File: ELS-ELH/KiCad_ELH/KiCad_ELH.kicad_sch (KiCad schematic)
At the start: 18 parts, among them J3 Screw_Terminal_01x12, J4 Screw_Terminal_01x02, J5 Screw_Terminal_01x02, J6 Screw_Terminal_01x02, J7 Screw_Terminal_01x02

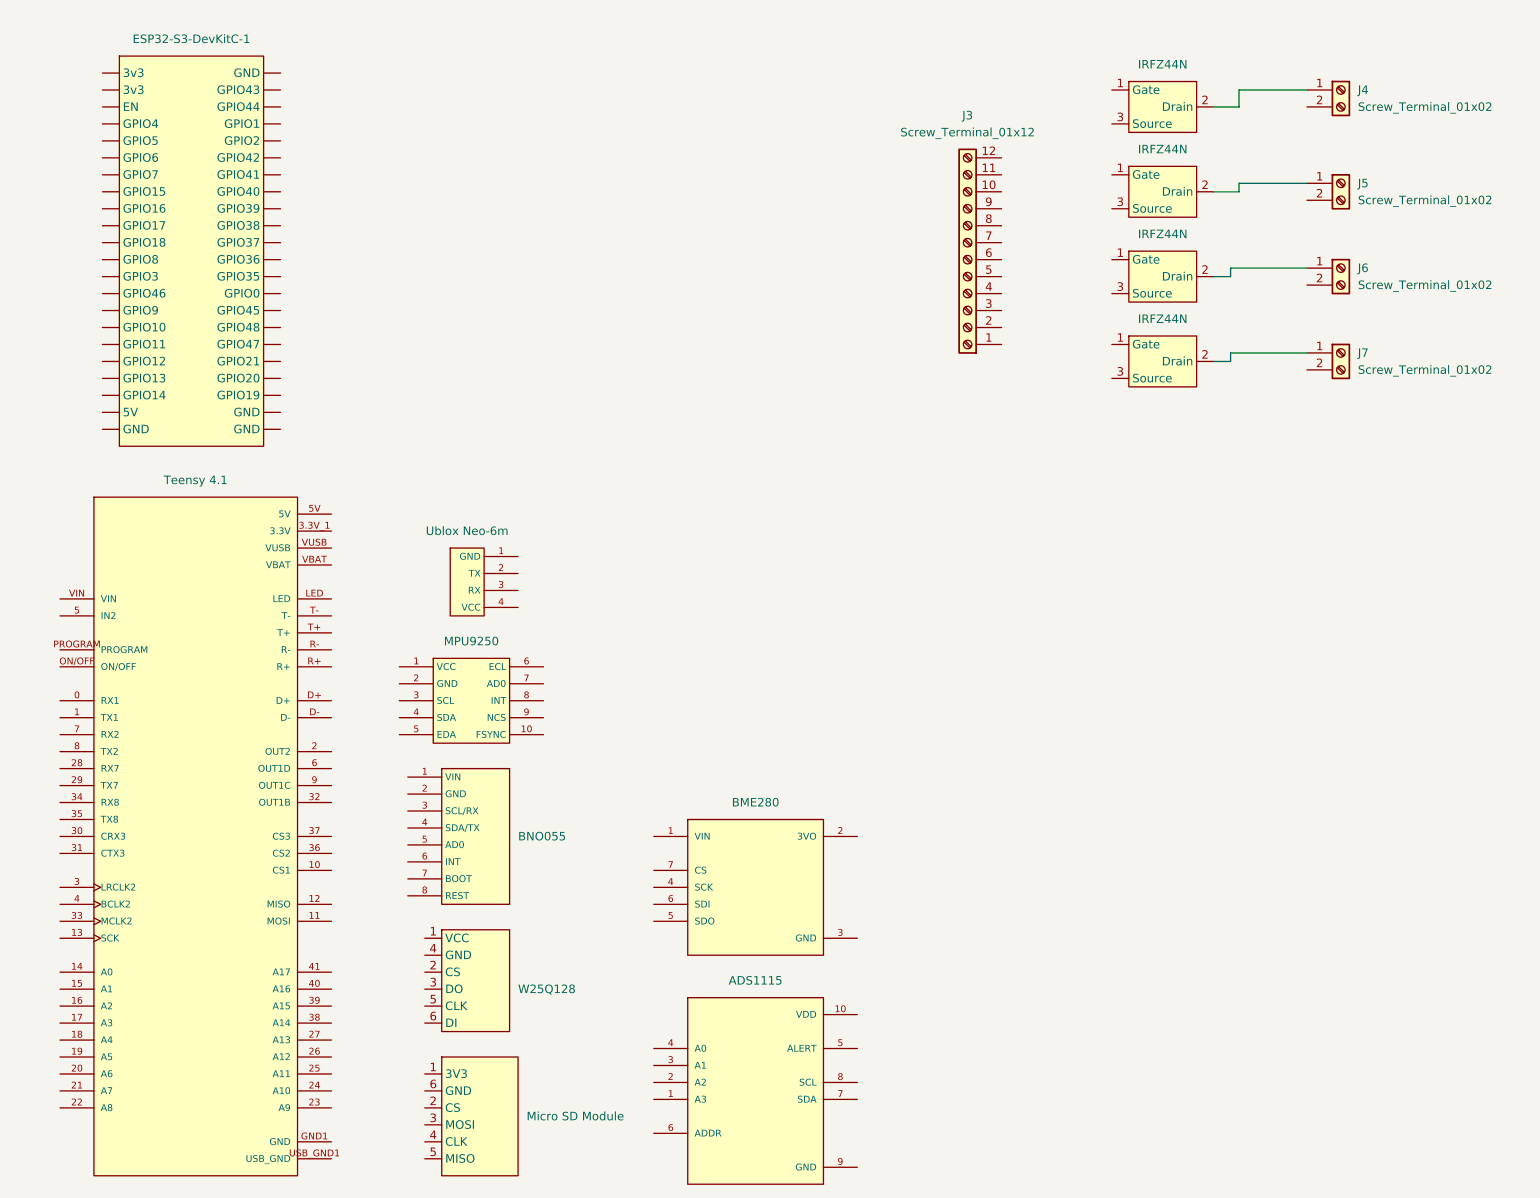
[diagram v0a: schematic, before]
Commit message: Some progress
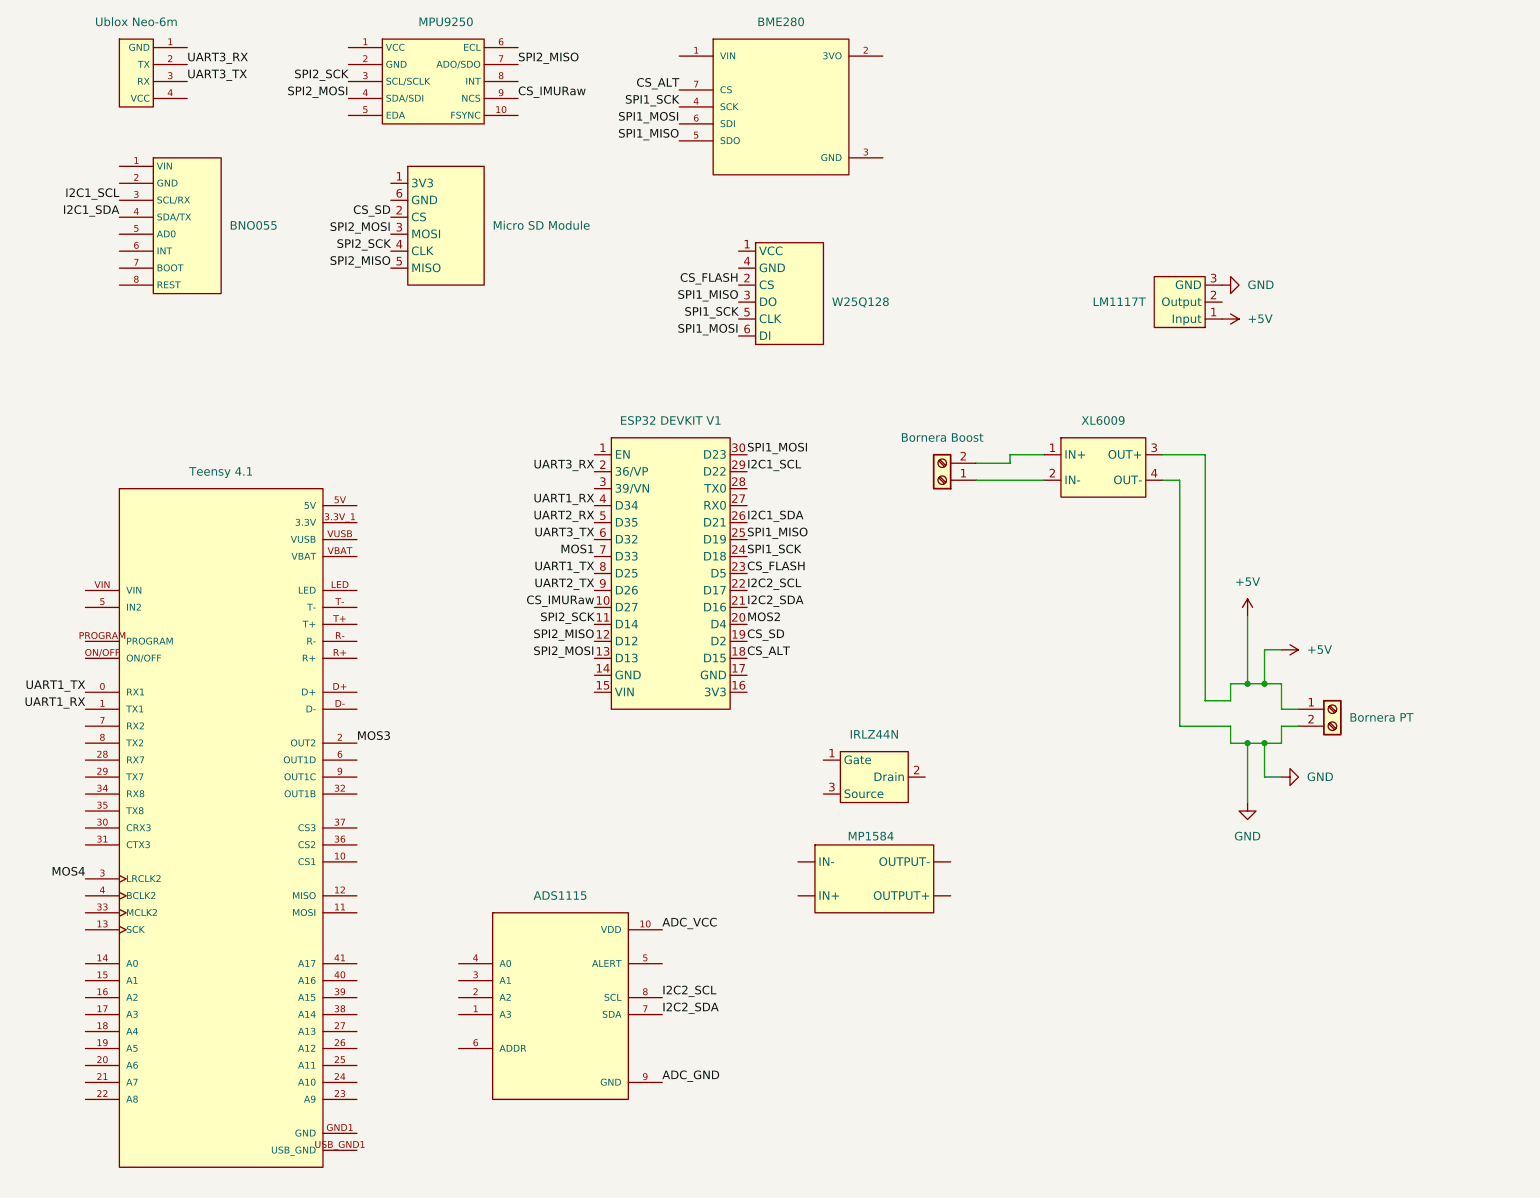
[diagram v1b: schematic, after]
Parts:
- removed ESP32-S3: ESP32-S3-DevKitC-1, ELH_Library:ESP32-S3-DevKitC-1, symbol ELH_Library:ESP32-S3-DevKitC-1
- removed J3: Screw_Terminal_01x12, symbol Connector:Screw_Terminal_01x12
- removed J4, J5, J6, J7: Screw_Terminal_01x02, symbol Connector:Screw_Terminal_01x02
- removed MOSFET1, MOSFET2, MOSFET3, MOSFET5: IRFZ44N, symbol ELH_Library:IRFZ44N
- added BOOST1: XL6009, ELH_Library:XL6009 Boost, symbol ELH_Library:XL6009_Boost
- added Bornera1: Bornera Boost, ELH_Library:Bornera 2P, symbol Connector:Screw_Terminal_01x02
- added Bornera2: Bornera PT, ELH_Library:Bornera 2P, symbol Connector:Screw_Terminal_01x02
- added ESP1: ESP32 DEVKIT V1, ELH_Library:ESP32 DEVKIT V1, symbol ELH_Library:ESP32 DEVKIT V1
- added MOSFET1: IRLZ44N, ELH_Library:IRLZ44N, symbol ELH_Library:IRFZ44N_1
- added Regulator1: LM1117T, symbol ELH_Library:LM1117T
- added Regulator3: MP1584, symbol ELH_Library:MP1584
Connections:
- net GND: now also BOOST1.4 (OUT-), Bornera2.2 (Pin_2), Regulator1.3 (GND)
- net SPI2_SCK: now reaches IMU1.3 (SCL/SCLK)
- net SPI2_SCK: now also SD_Adapter1.4 (CLK), ESP1.11 (D14)
- net SPI2_MOSI: now reaches IMU1.4 (SDA/SDI)
- net SPI2_MOSI: now also SD_Adapter1.3 (MOSI), ESP1.13 (D13)
- net SPI2_MISO: now reaches IMU1.7 (ADO/SDO)
- net SPI2_MISO: now also SD_Adapter1.5 (MISO), ESP1.12 (D12)
- net CS_IMURaw: now reaches IMU1.9 (NCS)
- net CS_IMURaw: now also ESP1.10 (D27)
- net UART3_RX: now reaches GPS1.2 (TX)
- net UART3_RX: now also ESP1.2 (36/VP)
- net UART3_TX: now reaches GPS1.3 (RX)
- net UART3_TX: now also ESP1.6 (D32)
- net UART1_TX: now reaches Teensy3.0 (RX1)
- net UART1_TX: now also ESP1.8 (D25)
- net UART1_RX: now reaches Teensy3.1 (TX1)
- net UART1_RX: now also ESP1.4 (D34)
- net MOS3: now reaches Teensy3.2 (OUT2)
- net MOS4: now reaches Teensy3.3 (LRCLK2)
- net CS_FLASH: now reaches W25QXX1.2 (CS)
- net CS_FLASH: now also ESP1.23 (D5)
- net SPI1_MISO: now reaches W25QXX1.3 (DO)
- net SPI1_MISO: now also BME2.5 (SDO), ESP1.25 (D19)
- net SPI1_SCK: now reaches W25QXX1.5 (CLK)
- net SPI1_SCK: now also BME2.4 (SCK), ESP1.24 (D18)
- net SPI1_MOSI: now reaches W25QXX1.6 (DI)
- net SPI1_MOSI: now also BME2.6 (SDI), ESP1.30 (D23)
- net CS_SD: now reaches SD_Adapter1.2 (CS)
- net CS_SD: now also ESP1.19 (D2)
- net I2C1_SCL: now reaches IMU3.3 (SCL/RX)
- net I2C1_SCL: now also ESP1.29 (D22)
- net I2C1_SDA: now reaches IMU3.4 (SDA/TX)
- net I2C1_SDA: now also ESP1.26 (D21)
- net CS_ALT: now reaches BME2.7 (CS)
- net CS_ALT: now also ESP1.18 (D15)
- net ADC_VCC: now reaches ADC1.10 (VDD)
- net I2C2_SDA: now reaches ADC1.7 (SDA)
- net I2C2_SDA: now also ESP1.21 (D16)
- net I2C2_SCL: now reaches ADC1.8 (SCL)
- net I2C2_SCL: now also ESP1.22 (D17)
- net ADC_GND: now reaches ADC1.9 (GND)
- new net: BOOST1.1 (IN+), Bornera1.2 (Pin_2)
- new net: BOOST1.2 (IN-), Bornera1.1 (Pin_1)
- new net +5V: BOOST1.3 (OUT+), Bornera2.1 (Pin_1), Regulator1.1 (Input)
- new net MOS1: ESP1.7 (D33)
- new net MOS2: ESP1.20 (D4)
- new net UART2_RX: ESP1.5 (D35)
- new net UART2_TX: ESP1.9 (D26)
